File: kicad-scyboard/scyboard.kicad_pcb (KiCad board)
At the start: 2 copper layers, 144 x 96.5 mm, 55 parts

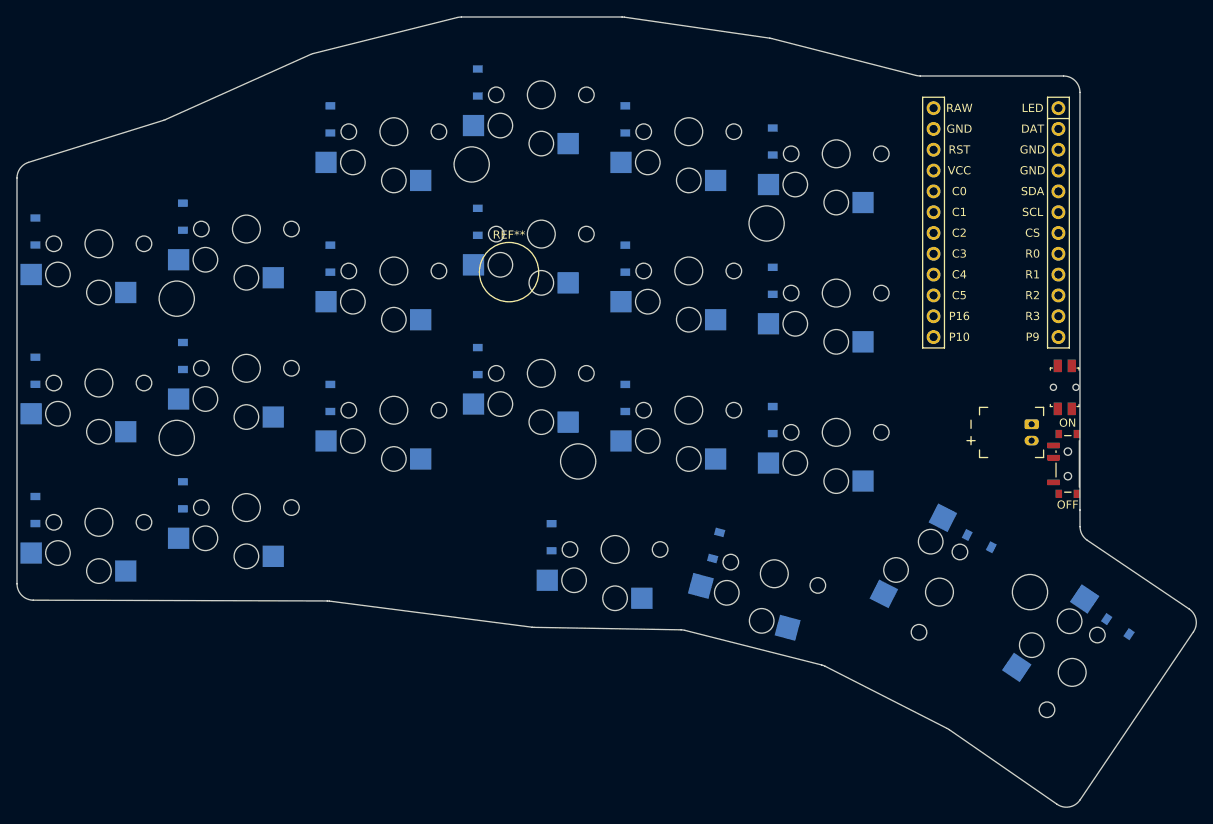
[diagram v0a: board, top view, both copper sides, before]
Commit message: Compile
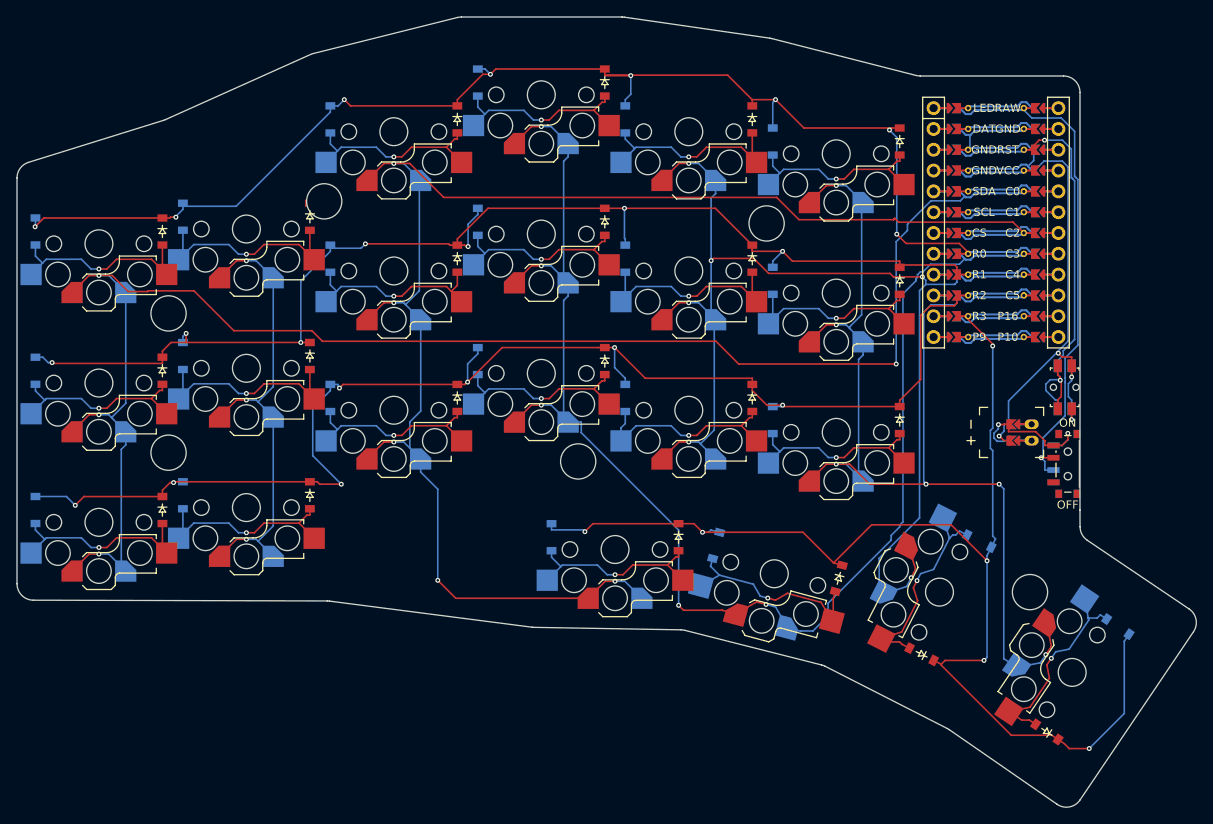
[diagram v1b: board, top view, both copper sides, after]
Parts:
- removed REF**: custom_case, custom:custom_case
- added D23: , ceoloide:diode_tht_sod123, F.Cu at (57.8, 98.5)
- added D24: , ceoloide:diode_tht_sod123, F.Cu at (57.8, 81.5)
- added D25: , ceoloide:diode_tht_sod123, F.Cu at (57.8, 64.5)
- added D26: , ceoloide:diode_tht_sod123, F.Cu at (75.8, 96.7)
- added D27: , ceoloide:diode_tht_sod123, F.Cu at (75.8, 79.7)
- added D28: , ceoloide:diode_tht_sod123, F.Cu at (75.8, 62.7)
- added D29: , ceoloide:diode_tht_sod123, F.Cu at (93.8, 84.8)
- added D30: , ceoloide:diode_tht_sod123, F.Cu at (93.8, 67.8)
- added D31: , ceoloide:diode_tht_sod123, F.Cu at (93.8, 50.8)
- added D32: , ceoloide:diode_tht_sod123, F.Cu at (111.8, 80.3)
- added D33: , ceoloide:diode_tht_sod123, F.Cu at (111.8, 63.3)
- added D34: , ceoloide:diode_tht_sod123, F.Cu at (111.8, 46.3)
- added D35: , ceoloide:diode_tht_sod123, F.Cu at (129.8, 84.8)
- added D36: , ceoloide:diode_tht_sod123, F.Cu at (129.8, 67.8)
- added D37: , ceoloide:diode_tht_sod123, F.Cu at (129.8, 50.8)
- added D38: , ceoloide:diode_tht_sod123, F.Cu at (147.8, 87.5)
- added D39: , ceoloide:diode_tht_sod123, F.Cu at (147.8, 70.5)
- added D40: , ceoloide:diode_tht_sod123, F.Cu at (147.8, 53.5)
- added D41: , ceoloide:diode_tht_sod123, F.Cu at (120.8, 101.8)
- added D42: , ceoloide:diode_tht_sod123, F.Cu at (140.3, 106.8)
- added D43: , ceoloide:diode_tht_sod123, F.Cu at (150.4, 116.1)
- added D44: , ceoloide:diode_tht_sod123, F.Cu at (165.7, 125.6)
- S1, S10, S11, S12, S13, S14, S15, S16, S17, S18, S19, S2, S20, S22, S3, S4, S5, S6, S7, S8, S9: footprint custom:custom_switch_choc_v1 -> ceoloide:switch_choc_v1_v2
- S21: footprint custom:custom_switch_choc_v1_1.5u -> ceoloide:switch_choc_v1_v2
- moved MH6 57.4 mm to (108.5, 92.6)
- moved MH5 55.3 mm to (163.7, 108.5)
- moved MH3 44.4 mm to (77.5, 60.8)
- moved MH4 36.7 mm to (131.5, 63.5)
- moved MH1 2.06 mm to (58.5, 74.5)
- moved MH2 2.06 mm to (58.5, 91.5)
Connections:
- JST1 pad 1: GND -> BAT_P
- JST1 pad 2: BAT_P -> GND
- MCU1 pad 1: LED -> MCU1_1
- MCU1 pad 10: R2 -> MCU1_10
- MCU1 pad 11: R3 -> MCU1_11
- MCU1 pad 12: P9 -> MCU1_12
- MCU1 pad 13: P10 -> MCU1_13
- MCU1 pad 14: P16 -> MCU1_14
- MCU1 pad 15: C5 -> MCU1_15
- MCU1 pad 16: C4 -> MCU1_16
- MCU1 pad 17: C3 -> MCU1_17
- MCU1 pad 18: C2 -> MCU1_18
- MCU1 pad 19: C1 -> MCU1_19
- MCU1 pad 2: DAT -> MCU1_2
- MCU1 pad 20: C0 -> MCU1_20
- MCU1 pad 21: VCC -> MCU1_21
- MCU1 pad 22: RST -> MCU1_22
- MCU1 pad 23: GND -> MCU1_23
- MCU1 pad 24: RAW -> MCU1_24
- MCU1 pad 3: GND -> MCU1_3
- MCU1 pad 4: GND -> MCU1_4
- MCU1 pad 5: SDA -> MCU1_5
- MCU1 pad 6: SCL -> MCU1_6
- MCU1 pad 7: CS -> MCU1_7
- MCU1 pad 8: R0 -> MCU1_8
- MCU1 pad 9: R1 -> MCU1_9
- PWR1 pad 1: (no net) -> BAT_P
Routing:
- net C0: track 0.00 -> 195.6 mm, vias 0 -> 4
- net C2: track 0.00 -> 191.2 mm, vias 0 -> 5
- net C3: track 0.00 -> 171.3 mm, vias 0 -> 5
- net R2: track 0.00 -> 170.3 mm, vias 0 -> 7
- net R0: track 0.00 -> 166.9 mm, vias 0 -> 8
- net R3: track 0.00 -> 162.5 mm, vias 0 -> 6
- net R1: track 0.00 -> 159.2 mm, vias 0 -> 7
- net C4: track 0.00 -> 149.0 mm, vias 0 -> 6
- net C5: track 0.00 -> 146.9 mm, vias 0 -> 6
- net GND: track 0.00 -> 91.1 mm, vias 0 -> 4
- net C1: track 0.00 -> 66.8 mm, vias 0 -> 3
- net RAW: track 0.00 -> 64.0 mm, vias 0 -> 1
- net RST: track 0.00 -> 57.2 mm, vias 0 -> 2
- net space_cluster_B: track 0.00 -> 25.5 mm, vias 0 -> 1
- net layer_cluster_B: track 0.00 -> 25.5 mm, vias 0 -> 1
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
